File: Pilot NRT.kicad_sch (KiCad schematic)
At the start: 71 parts, among them J1 Touchscreen, J10 Conn_01x02, J11 Conn_01x02, J12 Conn_01x02, J13 3.5'' LCD, J14 USB_B_Micro, J2 Conn_01x02, J3 Conn_01x02, J4 Conn_01x02, J5 Conn_01x02, J6 Conn_01x02, J7 Conn_01x02, J8 Conn_01x02, J9 Conn_01x02, SW1 SW_SPDT, SW2 SW_SPDT, U1 STM32F103CBT6, U2 W25X40CLSS, U3 AT24CS01-XHM, U4 USBLC6-2SC6, Y1 8MHz

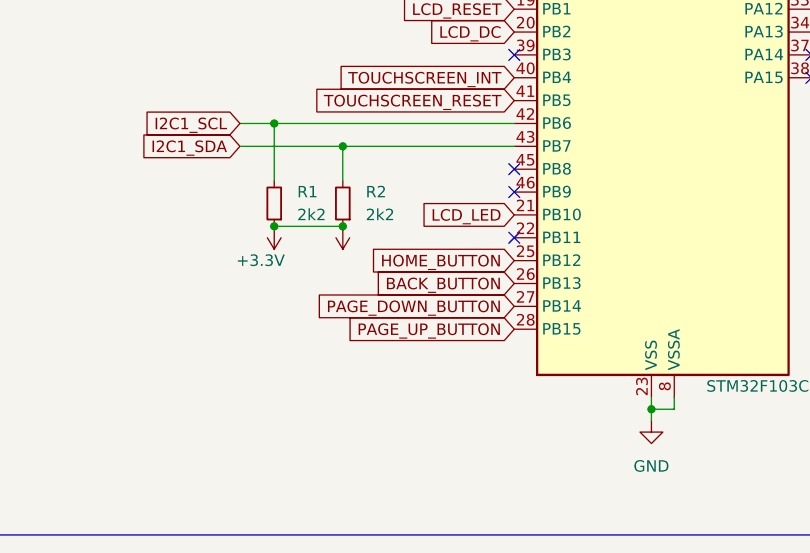
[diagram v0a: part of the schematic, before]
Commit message: rouch parts placement
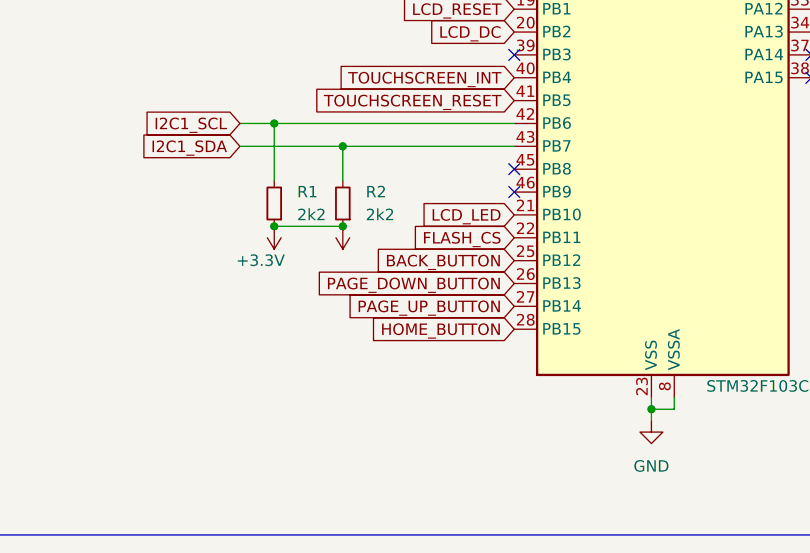
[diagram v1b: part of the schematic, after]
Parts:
- R24: footprint Resistor_SMD:R_0201_0603Metric -> flash_cs
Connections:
- net BACK_BUTTON: now also U1.25 (PB12); no longer U1.26 (PB13)
- net FLASH_CS: now also U1.22 (PB11)
- net HOME_BUTTON: now also U1.28 (PB15); no longer U1.25 (PB12)
- net PAGE_DOWN_BUTTON: now also U1.26 (PB13); no longer U1.27 (PB14)
- net PAGE_UP_BUTTON: now also U1.27 (PB14); no longer U1.28 (PB15)
- no-connect marks 9 -> 8
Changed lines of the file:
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@@
 	)
 	(no_connect
-		(at 71.12 163.83)
-	)
-	(no_connect
 		(at 266.7 135.89)
 	)
@@
 		)
 	)
-	(global_label "BACK_BUTTON"
-		(shape input)
-		(at 71.12 168.91 180)
-		(fields_autoplaced yes)
-		(effects
-			(font
-				(size 1.27 1.27)
-			)
-			(justify right)
-		)
-		(property "Intersheetrefs" "${INTERSHEET_REFS}"
-			(at 55.0719 168.91 0)
-			(effects
-				(font
-					(size 1.27 1.27)
-				)
-				(justify right)
-				(hide yes)
-			)
-		)
-	)
 	(global_label "LEFT_BUTTON"
 		(shape input)
@@
 		)
 	)
-	(global_label "PAGE_DOWN_BUTTON"
-		(shape input)
-		(at 71.12 171.45 180)
-		(fields_autoplaced yes)
-		(effects
-			(font
-				(size 1.27 1.27)
-			)
-			(justify right)
-		)
-		(property "Intersheetrefs" "${INTERSHEET_REFS}"
-			(at 48.8429 171.45 0)
-			(effects
-				(font
-					(size 1.27 1.27)
-				)
-				(justify right)
-				(hide yes)
-			)
-		)
-	)
 	(global_label "DOWN_BUTTON"
 		(shape input)
@@
 		)
 	)
-	(global_label "HOME_BUTTON"
+	(global_label "RIGHT_BUTTON"
 		(shape input)
-		(at 71.12 166.37 180)
+		(at 153.67 73.66 180)
 		(fields_autoplaced yes)
 		(effects
@@
 		)
 		(property "Intersheetrefs" "${INTERSHEET_REFS}"
-			(at 54.7091 166.37 0)
+			(at 137.0776 73.66 0)
 			(effects
 				(font
@@
 		)
 	)
-	(global_label "RIGHT_BUTTON"
+	(global_label "LCD_RESET"
 		(shape input)
-		(at 153.67 73.66 180)
+		(at 269.24 29.21 180)
 		(fields_autoplaced yes)
 		(effects
@@
 		)
 		(property "Intersheetrefs" "${INTERSHEET_REFS}"
-			(at 137.0776 73.66 0)
+			(at 255.974 29.21 0)
 			(effects
 				(font
@@
 		)
 	)
-	(global_label "LCD_RESET"
+	(global_label "OK_BUTTON"
 		(shape input)
-		(at 269.24 29.21 180)
+		(at 204.47 96.52 180)
 		(fields_autoplaced yes)
 		(effects
@@
 		)
 		(property "Intersheetrefs" "${INTERSHEET_REFS}"
-			(at 255.974 29.21 0)
+			(at 190.72 96.52 0)
 			(effects
 				(font
@@
 		)
 	)
-	(global_label "OK_BUTTON"
+	(global_label "USB1_CONN+"
 		(shape input)
-		(at 204.47 96.52 180)
+		(at 200.66 135.89 180)
 		(fields_autoplaced yes)
 		(effects
@@
 		)
 		(property "Intersheetrefs" "${INTERSHEET_REFS}"
-			(at 190.72 96.52 0)
+			(at 184.8538 135.89 0)
 			(effects
 				(font
@@
 		)
 	)
-	(global_label "USB1_CONN+"
+	(global_label "FLASH_CS"
 		(shape input)
-		(at 200.66 135.89 180)
+		(at 71.12 163.83 180)
 		(fields_autoplaced yes)
 		(effects
@@
 		)
 		(property "Intersheetrefs" "${INTERSHEET_REFS}"
-			(at 184.8538 135.89 0)
+			(at 58.9424 163.83 0)
 			(effects
 				(font
@@
 		)
 	)
+	(global_label "PAGE_UP_BUTTON"
+		(shape input)
+		(at 71.12 171.45 180)
+		(fields_autoplaced yes)
+		(effects
+			(font
+				(size 1.27 1.27)
+			)
+			(justify right)
+		)
+		(property "Intersheetrefs" "${INTERSHEET_REFS}"
+			(at 51.6248 171.45 0)
+			(effects
+				(font
+					(size 1.27 1.27)
+				)
+				(justify right)
+				(hide yes)
+			)
+		)
+	)
 	(global_label "TOUCHSCREEN_RESET"
 		(shape input)
@@
 		)
 	)
-	(global_label "PAGE_UP_BUTTON"
-		(shape input)
-		(at 71.12 173.99 180)
-		(fields_autoplaced yes)
-		(effects
-			(font
-				(size 1.27 1.27)
-			)
-			(justify right)
-		)
-		(property "Intersheetrefs" "${INTERSHEET_REFS}"
-			(at 51.6248 173.99 0)
-			(effects
-				(font
-					(size 1.27 1.27)
-				)
-				(justify right)
-				(hide yes)
-			)
-		)
-	)
 	(global_label "ON_BUTTON"
 		(shape input)
@@
 		)
 	)
+	(global_label "BACK_BUTTON"
+		(shape input)
+		(at 71.12 166.37 180)
+		(fields_autoplaced yes)
+		(effects
+			(font
+				(size 1.27 1.27)
+			)
+			(justify right)
+		)
+		(property "Intersheetrefs" "${INTERSHEET_REFS}"
+			(at 55.0719 166.37 0)
+			(effects
+				(font
+					(size 1.27 1.27)
+				)
+				(justify right)
+				(hide yes)
+			)
+		)
+	)
 	(global_label "I2C1_SCL"
 		(shape input)
@@
 		)
 	)
+	(global_label "HOME_BUTTON"
+		(shape input)
+		(at 71.12 173.99 180)
+		(fields_autoplaced yes)
+		(effects
+			(font
+				(size 1.27 1.27)
+			)
+			(justify right)
+		)
+		(property "Intersheetrefs" "${INTERSHEET_REFS}"
+			(at 54.7091 173.99 0)
+			(effects
+				(font
+					(size 1.27 1.27)
+				)
+				(justify right)
+				(hide yes)
+			)
+		)
+	)
 	(global_label "I2C1_SDA"
 		(shape input)
@@
 		)
 	)
+	(global_label "PAGE_DOWN_BUTTON"
+		(shape input)
+		(at 71.12 168.91 180)
+		(fields_autoplaced yes)
+		(effects
+			(font
+				(size 1.27 1.27)
+			)
+			(justify right)
+		)
+		(property "Intersheetrefs" "${INTERSHEET_REFS}"
+			(at 48.8429 168.91 0)
+			(effects
+				(font
+					(size 1.27 1.27)
+				)
+				(justify right)
+				(hide yes)
+			)
+		)
+	)
 	(global_label "I2C1_SDA"
 		(shape input)
@@
 			)
 		)
-		(property "Footprint" "Resistor_SMD:R_0201_0603Metric"
+		(property "Footprint" "flash_cs"
 			(at 248.92 58.42 0)
 			(effects
